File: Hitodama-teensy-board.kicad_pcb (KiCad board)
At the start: 2 copper layers, 17 parts, among them J1 Conn_01x12_Male, U4 Teensy3.6

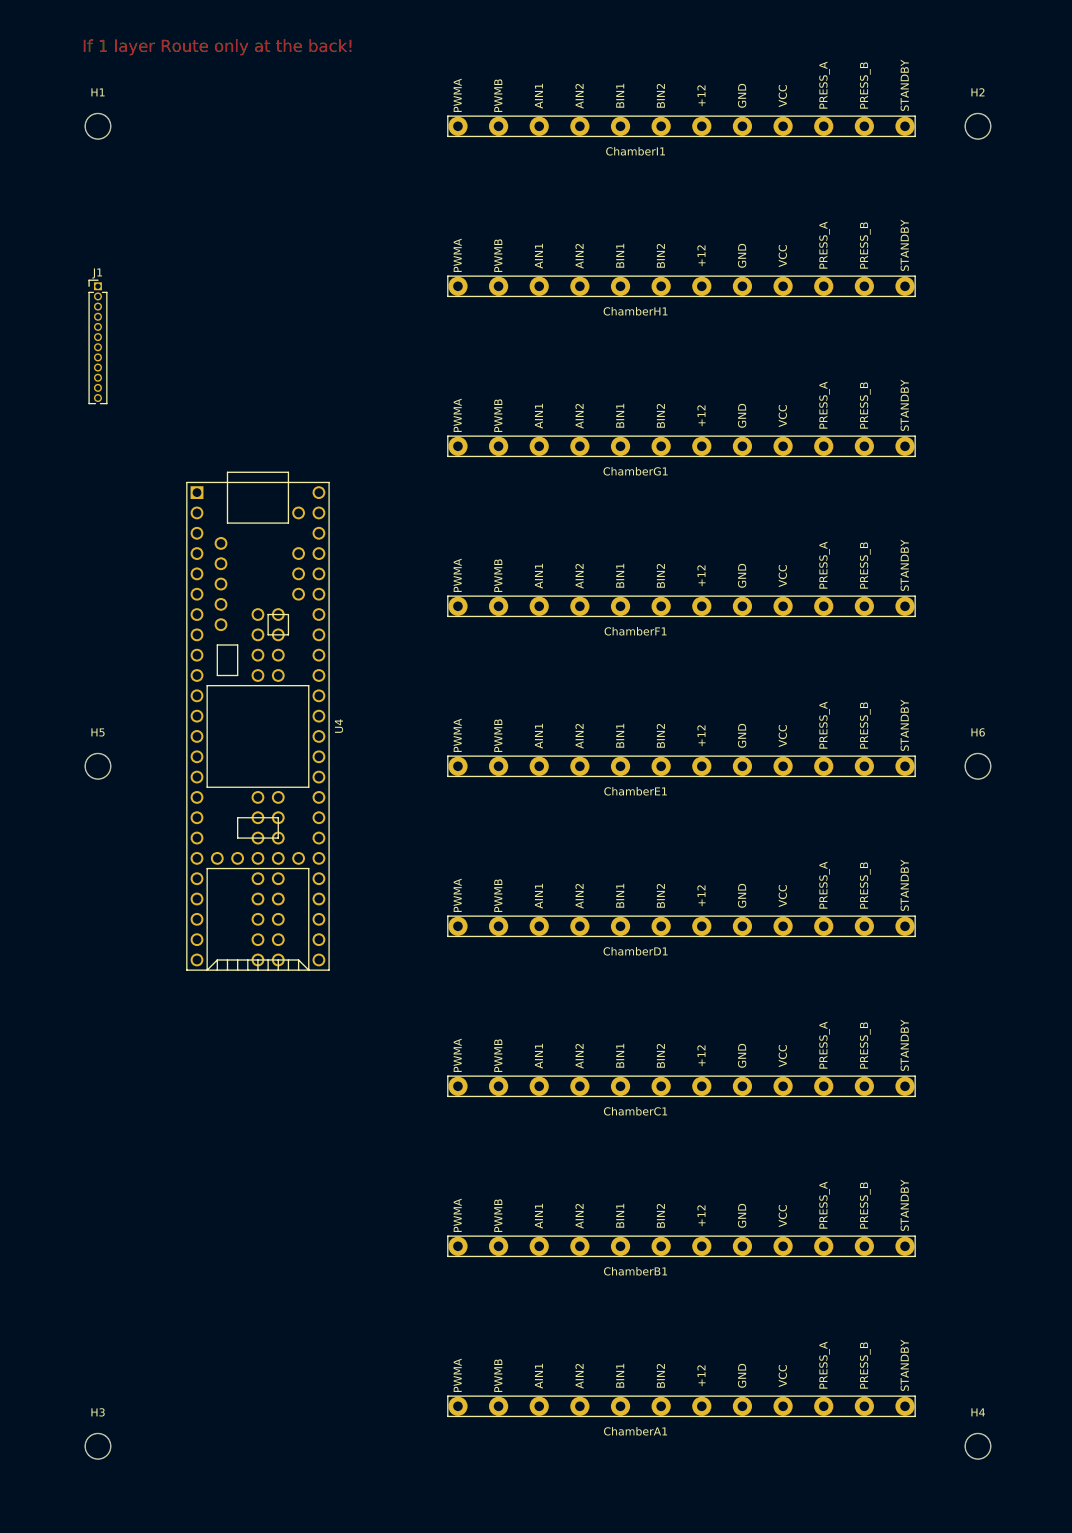
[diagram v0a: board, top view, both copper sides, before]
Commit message: (auto) routing
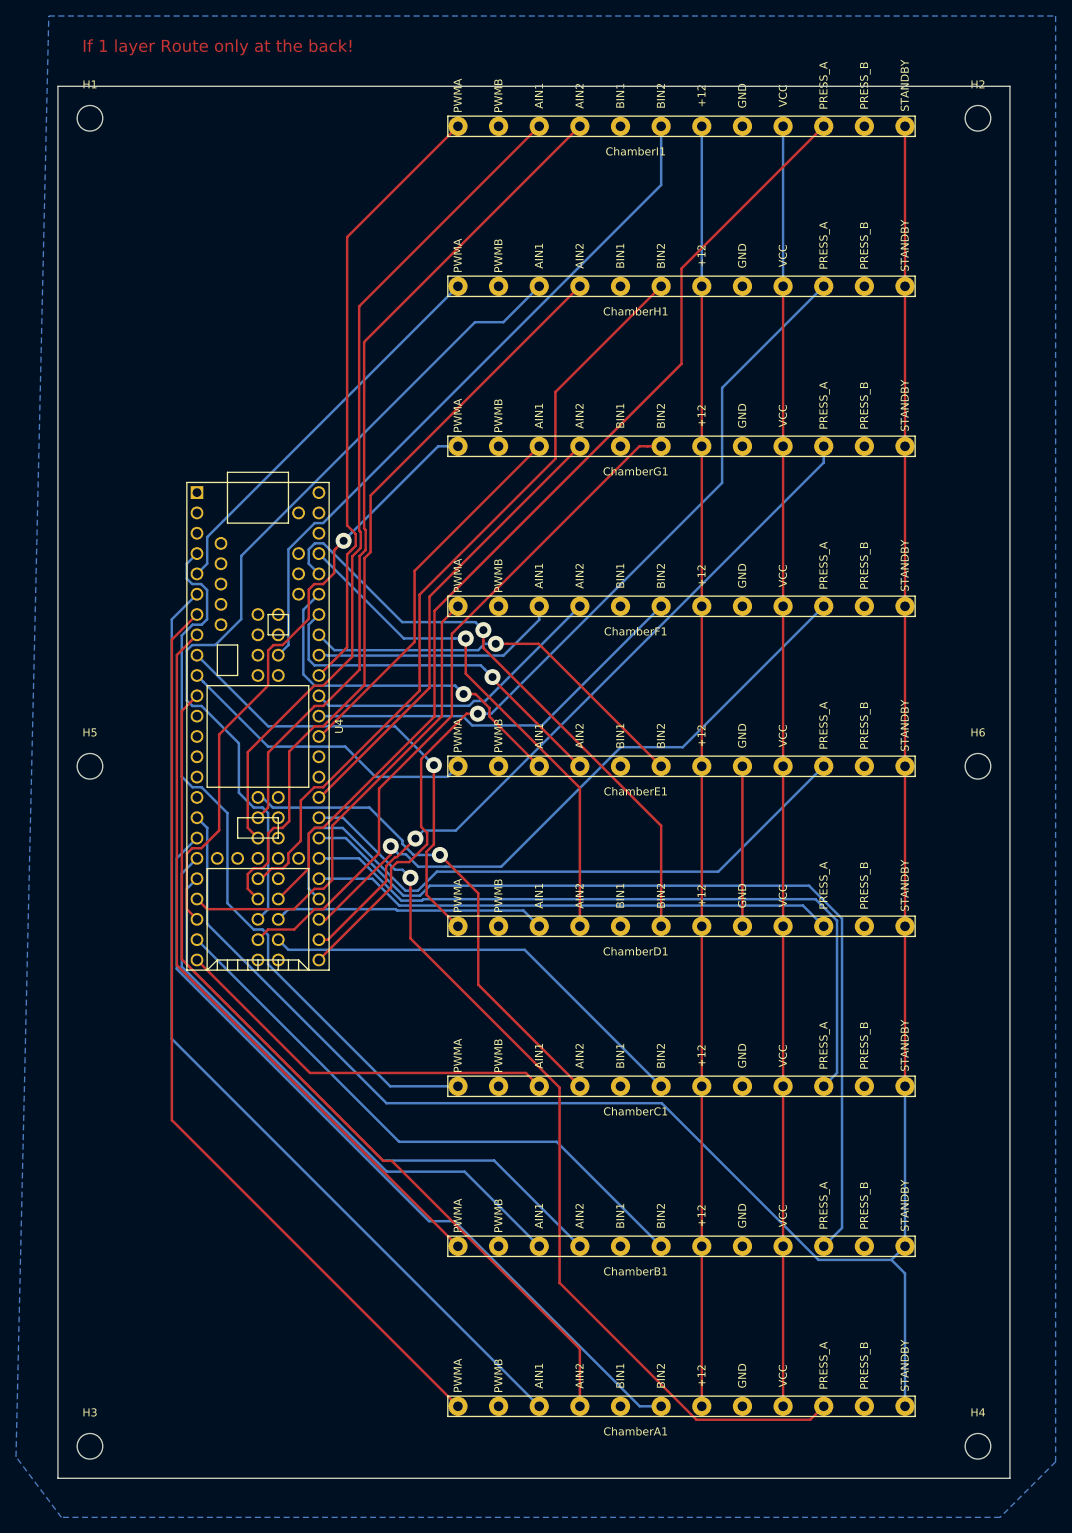
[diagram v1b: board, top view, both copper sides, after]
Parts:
- removed J1: Conn_01x12_Male, Connector_PinHeader_1.27mm:PinHeader_1x12_P1.27mm_Vertical
- moved H1 1.41 mm to (14.0, 14.0)
- moved H2 1.00 mm to (125.0, 14.0)
- moved H3 1.00 mm to (14.0, 180.0)
- moved H5 1.00 mm to (14.0, 95.0)
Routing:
- net /All.Stby: track 0.00 -> 278.1 mm
- net VCC: track 0.00 -> 160.0 mm
- net +12V: track 0.00 -> 160.0 mm
- net /ChamberI.ADC: track 0.00 -> 125.4 mm
- net /ChamberA.D1: track 0.00 -> 121.8 mm
- net /ChamberA.PWM: track 0.00 -> 115.1 mm
- net /ChamberA.ADC: track 0.00 -> 113.7 mm, vias 0 -> 1
- net /ChamberH.ADC: track 0.00 -> 113.7 mm, vias 0 -> 1
- net /ChamberB.ADC: track 0.00 -> 112.5 mm
- net /ChamberA.D2: track 0.00 -> 110.8 mm
- net /ChamberH.D1: track 0.00 -> 107.2 mm
- net /ChamberI.D1: track 0.00 -> 105.4 mm
- net /ChamberI.D2: track 0.00 -> 103.9 mm
- net /ChamberA.D3: track 0.00 -> 100.6 mm
- net /ChamberH.D3: track 0.00 -> 96.7 mm
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- added copper zone on B.Cu, net GND
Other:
- board outline added: 119 x 174 mm
- net class Default: clearance 0.2 -> 0.31; trace_width 0.25 -> 0.31; via_dia 0.8 -> 2; via_drill 0.4 -> 1
- rule trace_clearance: 0.2 -> 0.31
